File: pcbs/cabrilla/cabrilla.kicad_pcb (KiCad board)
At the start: 2 copper layers, 150 x 78 mm, 50 parts, among them J1 hm_1, J10 Conn_01x06, J11 Conn_01x08, J12 Conn_01x10, J2 hm_2, J3 hm_3, J4 hm_4, J5 conector_entradas, J6 UART_LCD, J7 leds_velocidad, J8 UART_lora, J9 Conn_01x08, U1 lorabee, U2 LCD, U3 LoRa, U4 AZ1117-3.3, Y1 lcd, Y2 LoRa

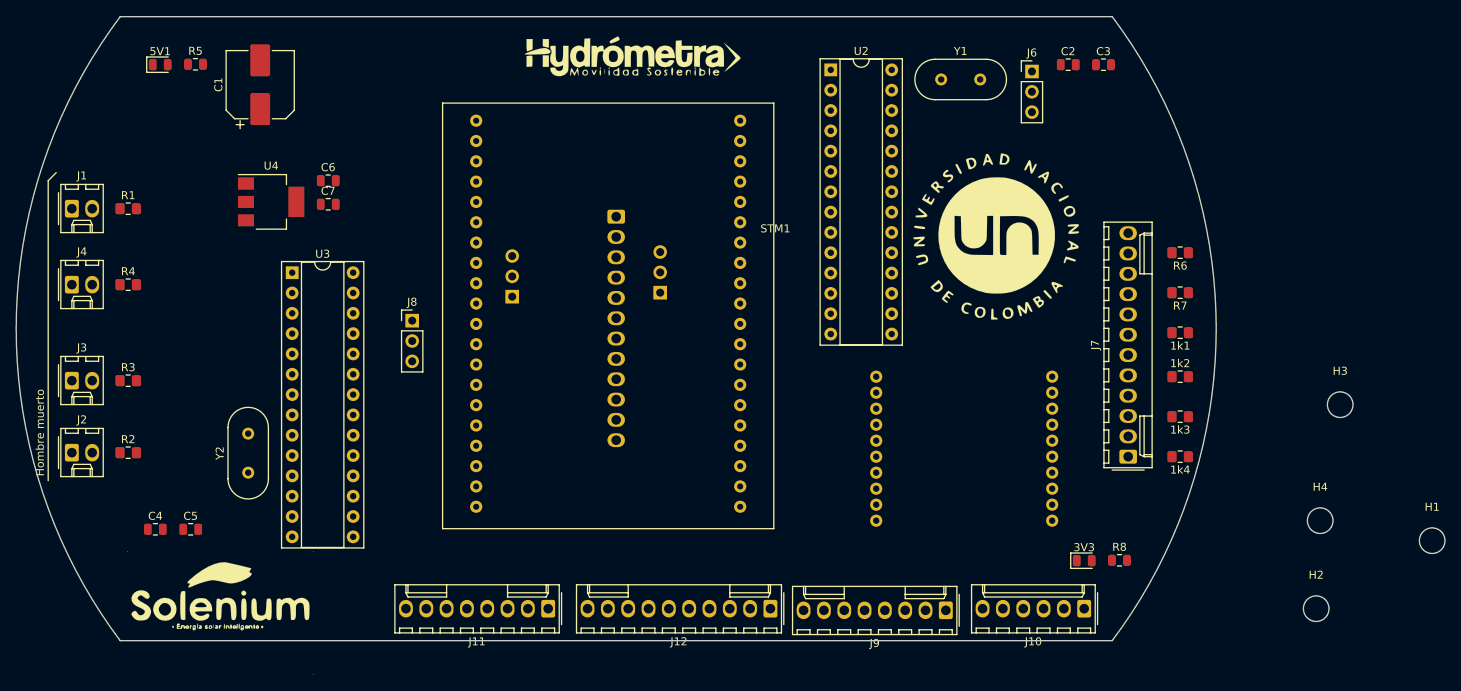
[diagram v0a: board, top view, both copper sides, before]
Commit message: PCB
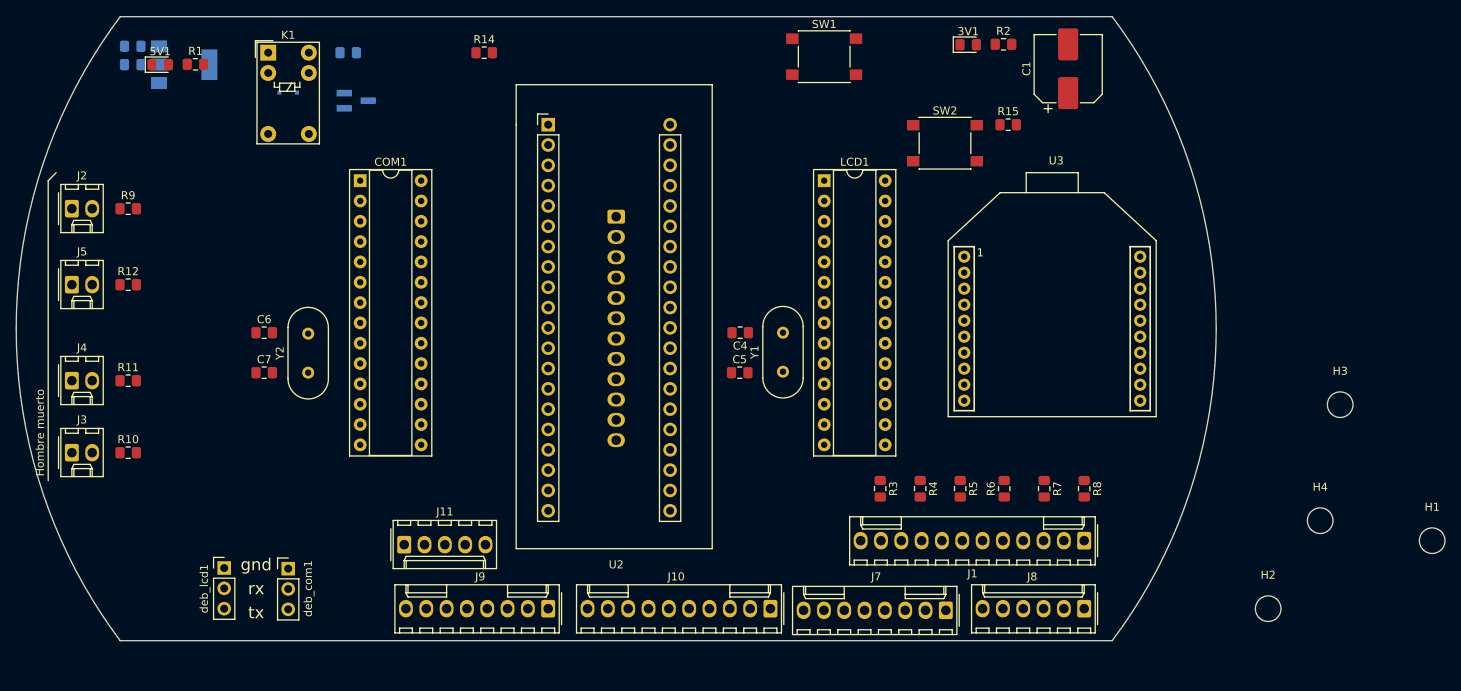
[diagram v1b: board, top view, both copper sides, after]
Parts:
- removed G***: LOGO, logos:hydro
- removed G***: LOGO, logos:id
- removed G***: LOGO, logos:un
- removed G***: LOGO, logos:solenium2
- removed JP1, JP2: jumper_con1, Connector_PinHeader_2.54mm:PinHeader_1x03_P2.54mm_Vertical
- removed STM1: u, arduino:STM32
- removed the U1 at (171.5, 103.0)
- added D1: 1N4148, Diode_SMD:D_SOD-323F, B.Cu at (98.0, 49.5)
- added J11: Conn_01x05, Connector_Molex:Molex_KK-254_AE-6410-05A_1x05_P2.54mm_Vertical, F.Cu at (112.5, 106.0)
- added K1: G5V-1, Relay_THT:Relay_SPDT_Omron_G5V-1, F.Cu at (95.5, 44.5)
- added Q1: PN2222A, Package_TO_SOT_SMD:SOT-23_Handsoldering, B.Cu at (106.5, 50.5)
- added R13: 10k, Resistor_SMD:R_0805_2012Metric_Pad1.15x1.40mm_HandSolder, B.Cu at (105.5, 44.5)
- added R14: 10k, Resistor_SMD:R_0805_2012Metric_Pad1.15x1.40mm_HandSolder, F.Cu at (122.5, 44.5)
- added R15: 10k, Resistor_SMD:R_0805_2012Metric_Pad1.15x1.40mm_HandSolder, F.Cu at (188.0, 53.5)
- added SW1: SW_Push, Button_Switch_SMD:SW_Push_1P1T_NO_6x6mm_H9.5mm, F.Cu at (165.0, 45.0)
- added SW2: SW_Push, Button_Switch_SMD:SW_Push_1P1T_NO_6x6mm_H9.5mm, F.Cu at (180.1, 55.8)
- added U2: STM32, elementos:STM32, F.Cu at (130.5, 53.5)
- added U3: lorabee, elementos:lorabee, F.Cu at (182.5, 70.0)
- 3V1: renamed from 3V3; footprint LED_SMD:LED_0805_2012Metric -> LED_SMD:LED_0805_2012Metric_Pad1.15x1.40mm_HandSolder
- 5V1: footprint LED_SMD:LED_0805_2012Metric -> LED_SMD:LED_0805_2012Metric_Pad1.15x1.40mm_HandSolder
- C2: renamed from C6; footprint Capacitor_SMD:C_0805_2012Metric -> Capacitor_SMD:C_0805_2012Metric_Pad1.15x1.40mm_HandSolder; moved to B.Cu
- C3: renamed from C7; footprint Capacitor_SMD:C_0805_2012Metric -> Capacitor_SMD:C_0805_2012Metric_Pad1.15x1.40mm_HandSolder; moved to B.Cu
- C4: renamed from C2; footprint Capacitor_SMD:C_0805_2012Metric -> Capacitor_SMD:C_0805_2012Metric_Pad1.15x1.40mm_HandSolder
- C5: renamed from C3; footprint Capacitor_SMD:C_0805_2012Metric -> Capacitor_SMD:C_0805_2012Metric_Pad1.15x1.40mm_HandSolder
- C6: renamed from C4; footprint Capacitor_SMD:C_0805_2012Metric -> Capacitor_SMD:C_0805_2012Metric_Pad1.15x1.40mm_HandSolder
- C7: renamed from C5; footprint Capacitor_SMD:C_0805_2012Metric -> Capacitor_SMD:C_0805_2012Metric_Pad1.15x1.40mm_HandSolder
- R1: renamed from R5; footprint Resistor_SMD:R_0805_2012Metric -> Resistor_SMD:R_0805_2012Metric_Pad1.15x1.40mm_HandSolder
- R2: renamed from R8; footprint Resistor_SMD:R_0805_2012Metric -> Resistor_SMD:R_0805_2012Metric_Pad1.15x1.40mm_HandSolder
- U1: renamed from U4; moved to B.Cu
- moved deb_lcd1 118.5 mm to (90.0, 108.9)
- moved C1 101.0 mm to (195.5, 46.5)
- moved 3V1 66.1 mm to (183.0, 43.5)
- moved R2 66.1 mm to (187.4, 43.5)
- moved C5 59.6 mm to (154.4, 84.5)
- moved C4 52.9 mm to (154.5, 79.5), turned to 180 degrees
- moved R3 47.7 mm to (172.0, 99.0), turned to 270 degrees
- moved Y1 41.5 mm to (159.8, 84.4), turned to 90 degrees
- moved R4 40.7 mm to (177.0, 99.0), turned to 270 degrees
- moved deb_com1 34.7 mm to (98.0, 109.0)
- moved R5 33.7 mm to (182.0, 99.0), turned to 270 degrees
- moved C3 30.0 mm to (78.6, 46.0), turned to 180 degrees
- moved C2 29.7 mm to (78.6, 43.7), turned to 180 degrees
- moved C6 28.1 mm to (95.0, 79.5)
- moved R6 26.1 mm to (187.5, 99.0), turned to 90 degrees
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- renumbered U3 to COM1, J7 to J1, J12 to J10, J1 to J2, J2 to J3, J3 to J4, J4 to J5, J5 to J6, J9 to J7, J10 to J8, J11 to J9, U2 to LCD1, R2 to R10, R3 to R11, R4 to R12, R6 to R3, R7 to R4, 1k1 to R5, 1k2 to R6, 1k3 to R7, 1k4 to R8, R1 to R9, J8 to deb_com1, J6 to deb_lcd1
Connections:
- net Net-(J5-Pad12) renamed /motor_h
- net Net-(J5-Pad9) renamed /freno
- COM1 pad 16: Net-(U3-Pad16) -> /Arduino LoRa/SS_lora
- COM1 pad 17: Net-(U3-Pad17) -> /Arduino LoRa/MOSI
- COM1 pad 18: Net-(U3-Pad18) -> /Arduino LoRa/MISO
- COM1 pad 19: Net-(U3-Pad19) -> /Arduino LoRa/SCK
- COM1 pad 2: /Arduino LoRa/rx_lora -> /tx_com
- COM1 pad 3: /Arduino LoRa/tx_lora -> /rx_com
- J2 pad 1: +5V -> +3V3
- J3 pad 1: +5V -> +3V3
- J4 pad 1: +5V -> +3V3
- J5 pad 1: +5V -> +3V3
- J6 pad 10: /com_1 -> Net-(J6-Pad10)
- J6 pad 11: /com_2 -> /motor_l
- J6 pad 2: +5V -> /vin
- J6 pad 7: /hm -> /pwm_motor
- J6 pad 8: /motor_out -> /reversa
- LCD1 pad 2: /Arduino LCD/rx_lcd -> /rx_lcd
- LCD1 pad 3: /Arduino LCD/tx_lcd -> /tx_lcd
- deb_com1 pad 2: /Arduino LoRa/tx_lora -> /tx_com
- deb_com1 pad 3: /Arduino LoRa/rx_lora -> /rx_com
- deb_lcd1 pad 2: /Arduino LCD/tx_lcd -> /rx_lcd
- deb_lcd1 pad 3: /Arduino LCD/rx_lcd -> /tx_lcd
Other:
- board text added: "gnd"
- board text added: "rx"
- board text added: "tx"
